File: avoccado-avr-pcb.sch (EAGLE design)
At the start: 32 parts, among them IC1 MCP1703CB, Q1 #MHz, Q2 MOSFET-NCHANNEL2N7002PW, U1 ATMEGA168#, U2 MCP73831, X1 Micro USB

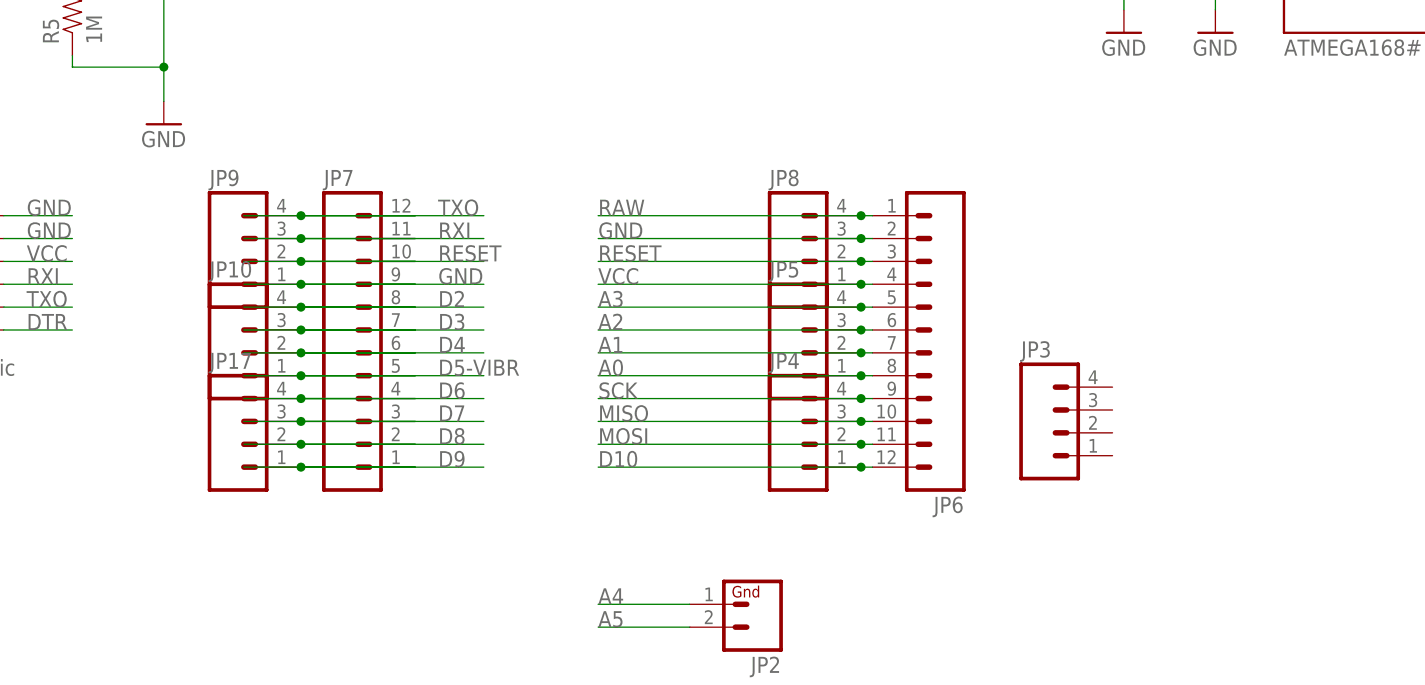
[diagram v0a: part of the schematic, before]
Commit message: evaluating SMD pads
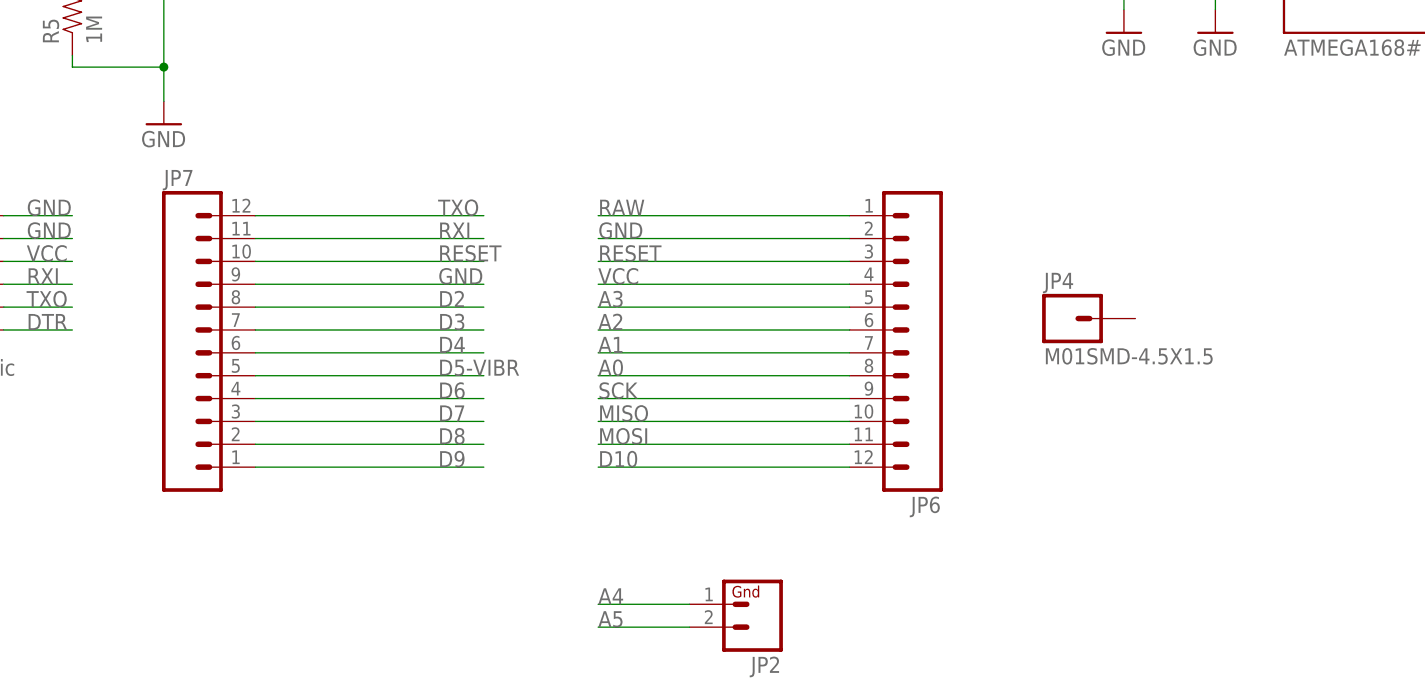
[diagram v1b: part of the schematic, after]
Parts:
- removed JP10, JP17, JP3, JP5, JP8, JP9: (no value), SparkFun-Connectors:M04SMD
- JP4: value (none) -> M01SMD-4.5X1.5; device SparkFun-Connectors:M04SMD -> SparkFun-Connectors:M01SMD-4.5X1.5
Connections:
- net A0: no longer JP5.1
- net A1: no longer JP5.2
- net A2: no longer JP5.3
- net A3: no longer JP5.4
- net D10: no longer JP4.1
- net D2: no longer JP10.4
- net D3: no longer JP10.3
- net D4: no longer JP10.2
- net D5-VIBR: no longer JP10.1
- net D6: no longer JP17.4
- net D7: no longer JP17.3
- net D8: no longer JP17.2
- net D9: no longer JP17.1
- net GND: no longer JP8.3, JP9.1
- net MISO: no longer JP4.3
- net MOSI: no longer JP4.2
- net RAW: no longer JP8.4
- net RESET: no longer JP8.2, JP9.2
- net RXI: no longer JP9.3
- net SCK: no longer JP4.4
- net TXO: no longer JP9.4
- net VCC: no longer JP8.1
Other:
- moved on the sheet: JP6, JP7
